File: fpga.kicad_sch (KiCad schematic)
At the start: 11 parts, among them U10 P0082_BOTTOMMOUNT, Y1 XLL735080.000000I

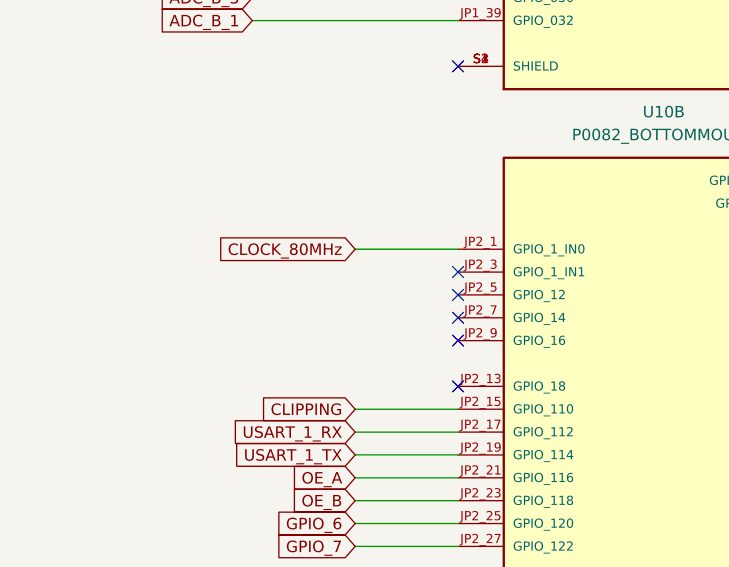
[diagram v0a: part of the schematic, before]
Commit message: Do most of the PCB
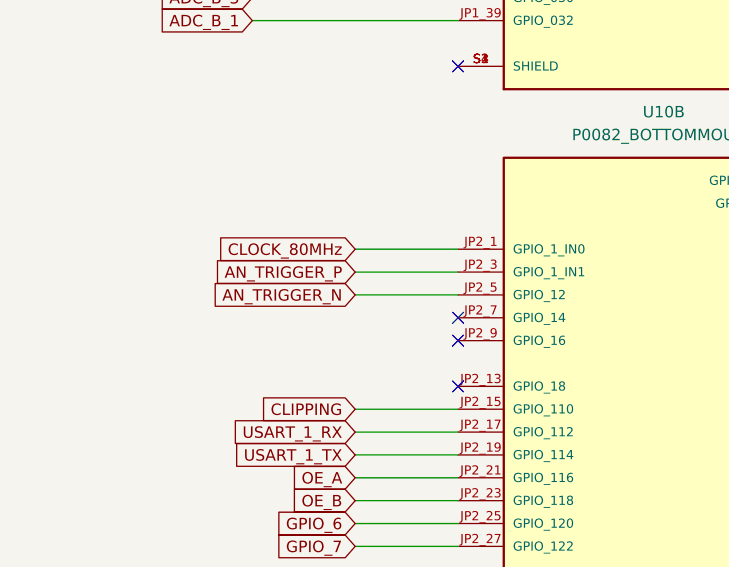
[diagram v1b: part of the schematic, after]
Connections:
- net AN_TRIGGER_P: now reaches U10.JP2_3 (GPIO_1_IN1)
- net AN_TRIGGER_N: now reaches U10.JP2_5 (GPIO_12)
- no-connect marks 21 -> 19
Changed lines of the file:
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@@
-	)
-	(no_connect
-		(at 80.01 125.73)
 	)
 	(no_connect
@@
 	)
 	(no_connect
-		(at 80.01 123.19)
-	)
-	(no_connect
 		(at 125.73 138.43)
 	)
@@
 	(wire
 		(pts
+			(xy 68.58 125.73) (xy 80.01 125.73)
+		)
+		(stroke
+			(width 0)
+			(type default)
+		)
+	)
+	(wire
+		(pts
 			(xy 127 175.26) (xy 127 179.07)
 		)
@@
 		(pts
 			(xy 232.41 85.09) (xy 232.41 87.63)
+		)
+		(stroke
+			(width 0)
+			(type default)
+		)
+	)
+	(wire
+		(pts
+			(xy 68.58 123.19) (xy 80.01 123.19)
 		)
 		(stroke
@@
 		)
 	)
+	(global_label "AN_TRIGGER_N"
+		(shape input)
+		(at 68.58 125.73 180)
+		(fields_autoplaced yes)
+		(effects
+			(font
+				(size 1.27 1.27)
+			)
+			(justify right)
+		)
+		(property "Intersheetrefs" "${INTERSHEET_REFS}"
+			(at 52.1086 125.73 0)
+			(effects
+				(font
+					(size 1.27 1.27)
+				)
+				(justify right)
+				(hide yes)
+			)
+		)
+	)
 	(global_label "ADC_B_2"
 		(shape input)
@@
 				(hide yes)
 			)
+		)
+	)
+	(global_label "AN_TRIGGER_P"
+		(shape input)
+		(at 68.58 123.19 180)
+		(fields_autoplaced yes)
+		(effects
+			(font
+				(size 1.27 1.27)
+			)
+			(justify right)
+		)
+		(property "Intersheetrefs" "${INTERSHEET_REFS}"
+			(at 52.1691 123.19 0)
+			(effects
+				(font
+					(size 1.27 1.27)
+				)
+				(justify right)
+				(hide yes)
+			)
